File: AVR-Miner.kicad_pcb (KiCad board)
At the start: 2 copper layers, 20 x 30 mm, 17 parts, among them J1 EXP, J2 AVR-ISP-6, SW1 RESET, U1 ATmega328P-AU, Y1 16MHz

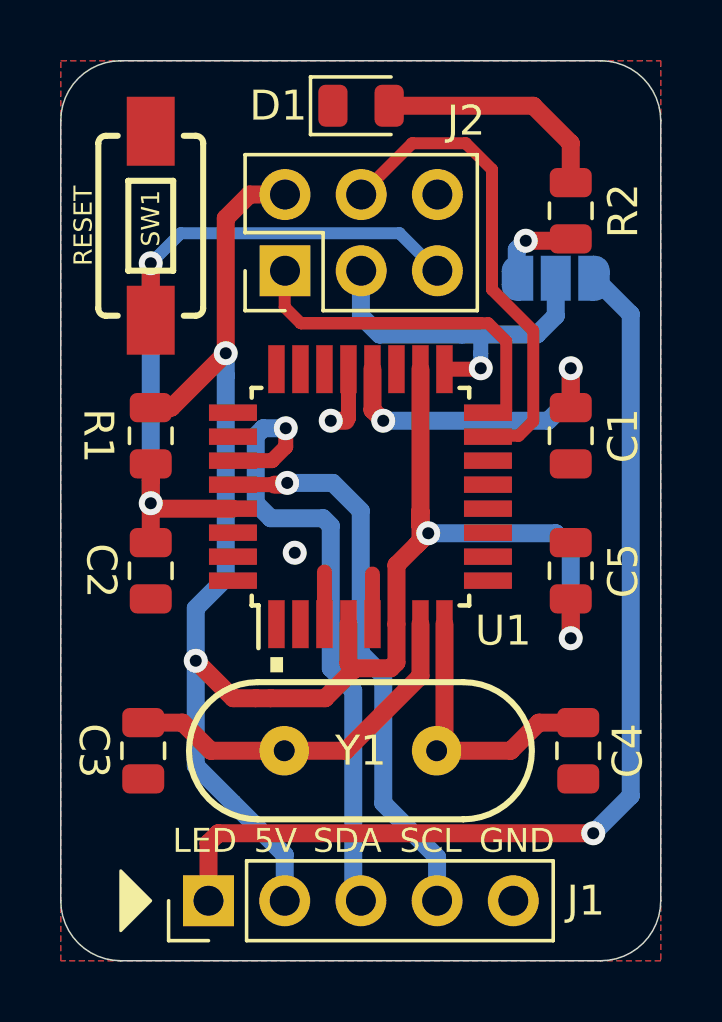
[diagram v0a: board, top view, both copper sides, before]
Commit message: Updated project files for KiCad 7 & Added Gerber files
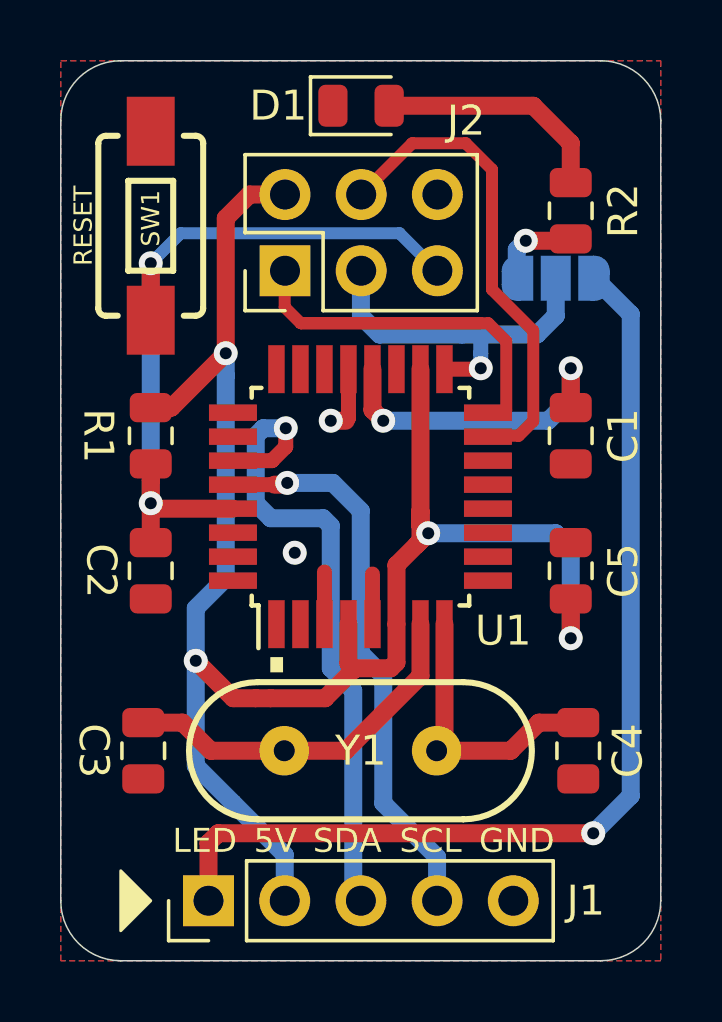
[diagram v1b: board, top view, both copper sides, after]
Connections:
- U1 pad 1: Net-(U1-Pad1) -> unconnected-(U1-PD3-Pad1)
- U1 pad 10: Net-(U1-Pad10) -> unconnected-(U1-PD6-Pad10)
- U1 pad 11: Net-(U1-Pad11) -> unconnected-(U1-PD7-Pad11)
- U1 pad 12: Net-(U1-Pad12) -> unconnected-(U1-PB0-Pad12)
- U1 pad 13: Net-(U1-Pad13) -> unconnected-(U1-PB1-Pad13)
- U1 pad 14: Net-(U1-Pad14) -> unconnected-(U1-PB2-Pad14)
- U1 pad 19: Net-(U1-Pad19) -> unconnected-(U1-ADC6-Pad19)
- U1 pad 2: Net-(U1-Pad2) -> unconnected-(U1-PD4-Pad2)
- U1 pad 22: Net-(U1-Pad22) -> unconnected-(U1-ADC7-Pad22)
- U1 pad 23: Net-(U1-Pad23) -> unconnected-(U1-PC0-Pad23)
- U1 pad 24: Net-(U1-Pad24) -> unconnected-(U1-PC1-Pad24)
- U1 pad 25: Net-(U1-Pad25) -> unconnected-(U1-PC2-Pad25)
- U1 pad 26: Net-(U1-Pad26) -> unconnected-(U1-PC3-Pad26)
- U1 pad 30: Net-(U1-Pad30) -> unconnected-(U1-PD0-Pad30)
- U1 pad 31: Net-(U1-Pad31) -> unconnected-(U1-PD1-Pad31)
- U1 pad 32: Net-(U1-Pad32) -> unconnected-(U1-PD2-Pad32)
- U1 pad 9: Net-(U1-Pad9) -> unconnected-(U1-PD5-Pad9)
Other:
- net class Default removed
